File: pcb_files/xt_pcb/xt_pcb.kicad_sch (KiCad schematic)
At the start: 36 parts, among them J1 Conn_01x04_Socket, J2 Conn_01x05, J3 USB_C_Receptacle_USB2.0, U1 XC6206PxxxMR, U2 RP2040, U3 W25Q128JVS, U4 SRV05-4, Y1 Crystal_GND24

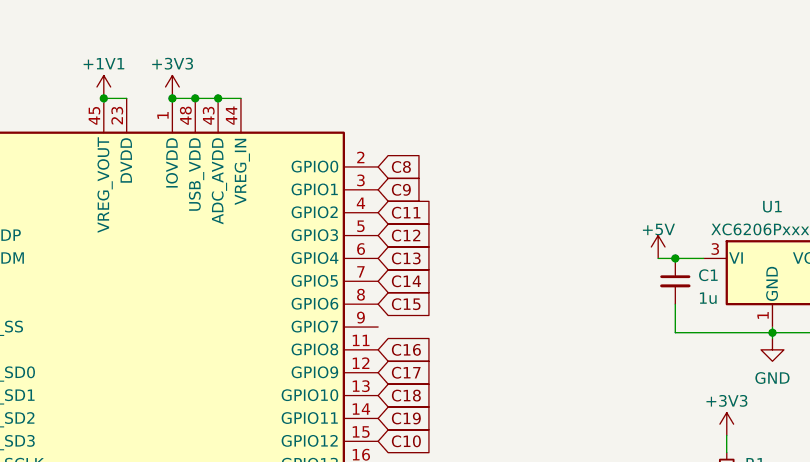
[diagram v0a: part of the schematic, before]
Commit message: tweaks
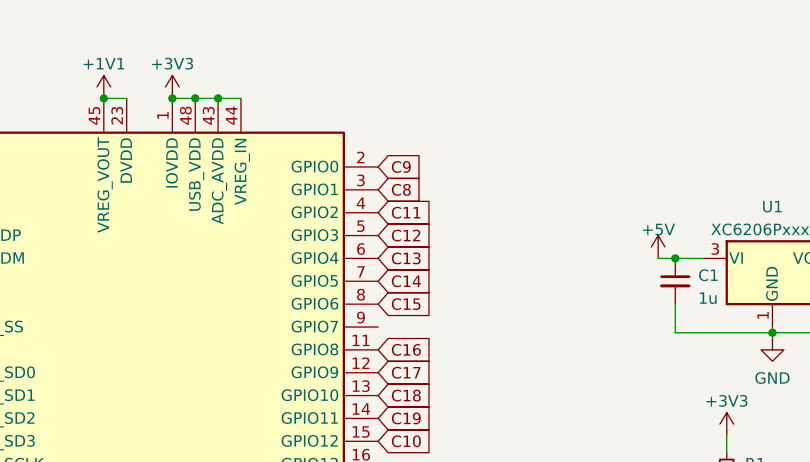
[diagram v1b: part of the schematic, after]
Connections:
- net C8: now also U2.3 (GPIO1); no longer U2.2 (GPIO0)
- net C9: now also U2.2 (GPIO0); no longer U2.3 (GPIO1)

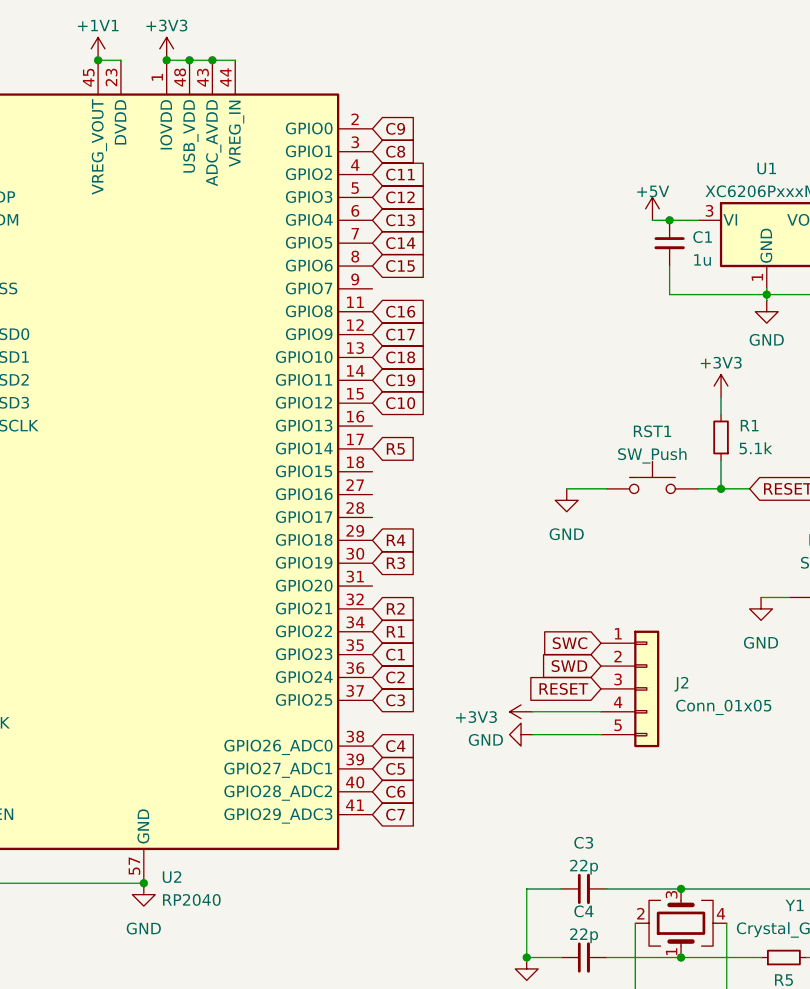
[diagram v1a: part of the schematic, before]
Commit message: vias removed
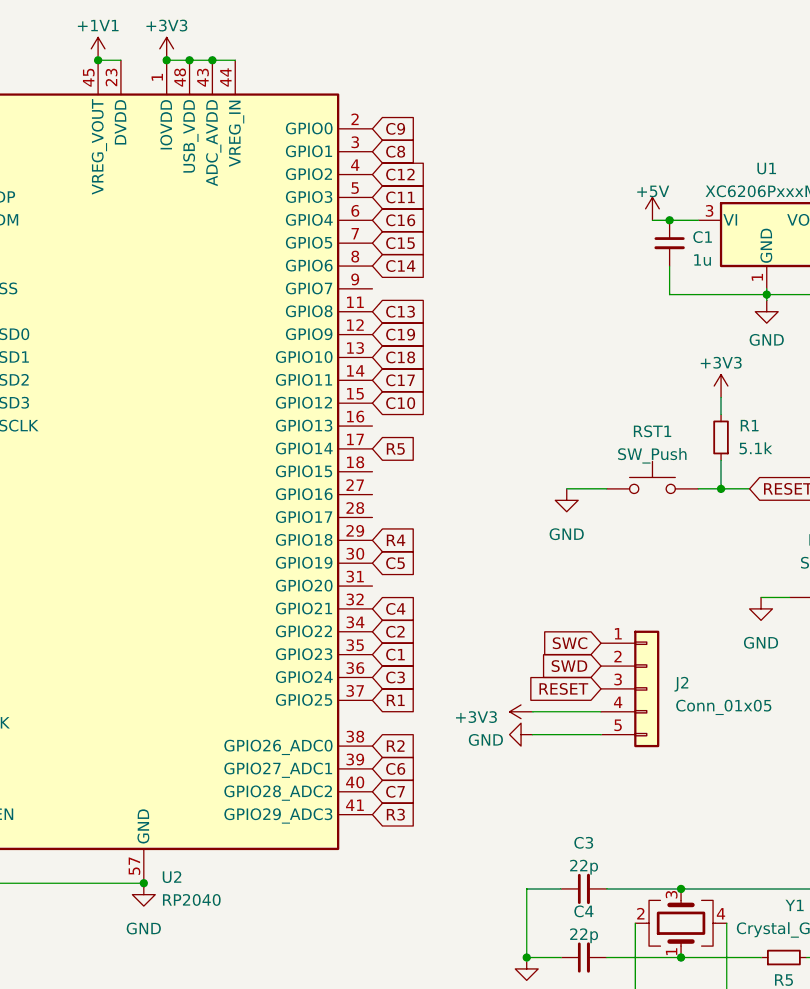
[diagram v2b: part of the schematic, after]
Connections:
- net C11: now also U2.5 (GPIO3); no longer U2.4 (GPIO2)
- net C12: now also U2.4 (GPIO2); no longer U2.5 (GPIO3)
- net C13: now also U2.11 (GPIO8); no longer U2.6 (GPIO4)
- net C14: now also U2.8 (GPIO6); no longer U2.7 (GPIO5)
- net C15: now also U2.7 (GPIO5); no longer U2.8 (GPIO6)
- net C16: now also U2.6 (GPIO4); no longer U2.11 (GPIO8)
- net C17: now also U2.14 (GPIO11); no longer U2.12 (GPIO9)
- net C19: now also U2.12 (GPIO9); no longer U2.14 (GPIO11)
- net C2: now also U2.34 (GPIO22); no longer U2.36 (GPIO24)
- net C3: now also U2.36 (GPIO24); no longer U2.37 (GPIO25)
- net C4: now also U2.32 (GPIO21); no longer U2.38 (GPIO26_ADC0)
- net C5: now also U2.30 (GPIO19); no longer U2.39 (GPIO27_ADC1)
- net C6: now also U2.39 (GPIO27_ADC1); no longer U2.40 (GPIO28_ADC2)
- net C7: now also U2.40 (GPIO28_ADC2); no longer U2.41 (GPIO29_ADC3)
- net R1: now also U2.37 (GPIO25); no longer U2.34 (GPIO22)
- net R2: now also U2.38 (GPIO26_ADC0); no longer U2.32 (GPIO21)
- net R3: now also U2.41 (GPIO29_ADC3); no longer U2.30 (GPIO19)
